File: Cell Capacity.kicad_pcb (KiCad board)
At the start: 2 copper layers, 84.5 x 80.5 mm, 24 parts, among them Q1 IRLZ44N, SW1 SW_Push, SW2 SW_Push, U1 LM358

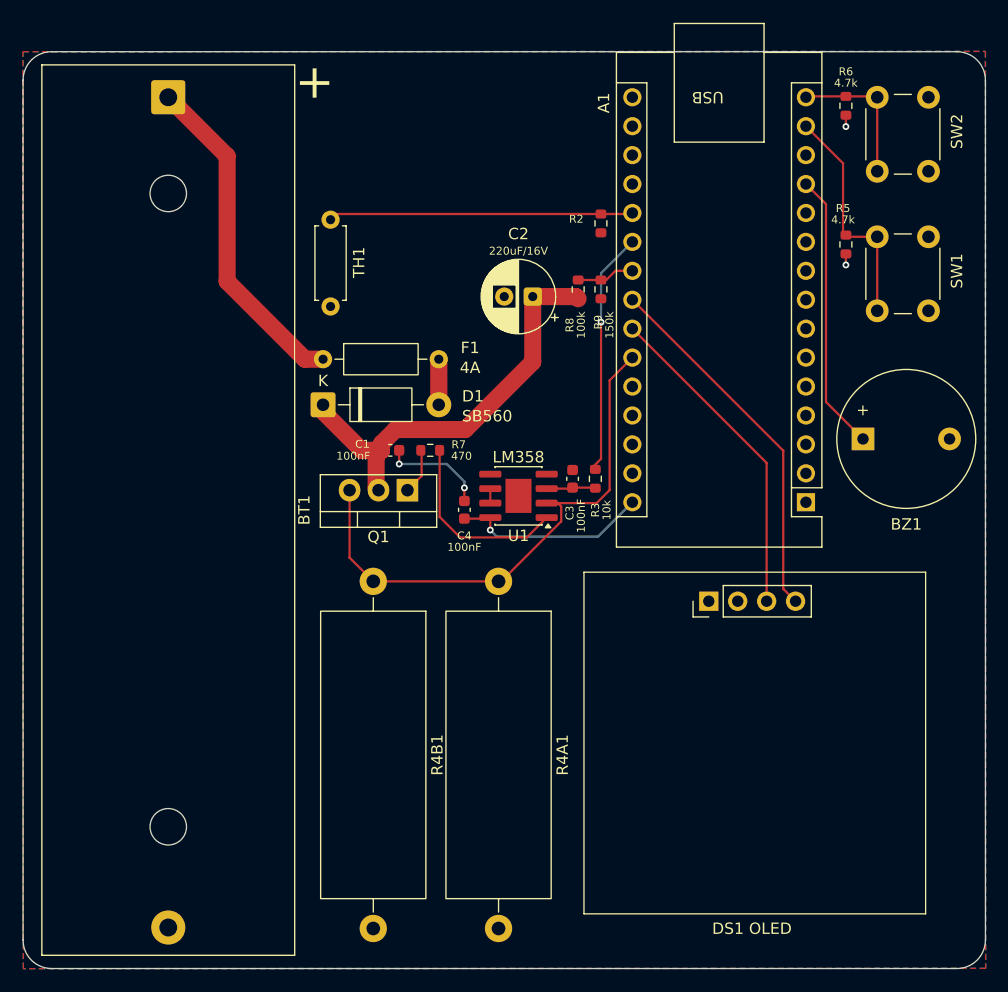
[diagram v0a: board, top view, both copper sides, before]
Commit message: layout iter2
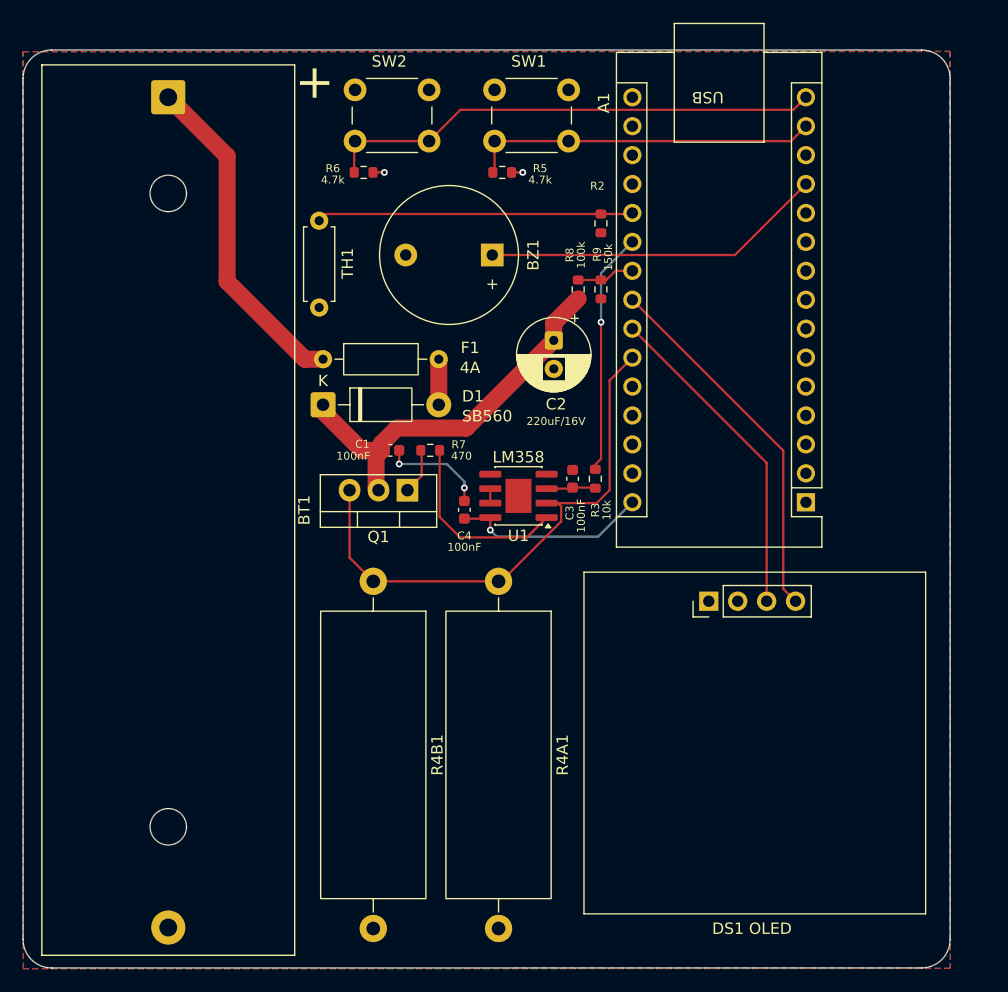
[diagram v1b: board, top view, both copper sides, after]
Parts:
- moved R6 42.8 mm to (94.9, 59.4), turned to 180 degrees
- moved SW2 39.4 mm to (100.7, 56.6), turned to 180 degrees
- moved BZ1 36.3 mm to (106.2, 66.6), turned to 180 degrees
- moved SW1 30.9 mm to (112.9, 56.6), turned to 180 degrees
- moved R5 30.8 mm to (107.1, 59.4), turned to 180 degrees
- moved C2 4.27 mm to (111.6, 74.1), turned to -90 degrees
- moved TH1 1.00 mm to (91.0, 71.2)
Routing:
- net /DOWN: track 12.7 -> 44.0 mm
- net /UP/START: track 20.3 -> 31.0 mm
- net /BUZZ: track 24.5 -> 30.1 mm
- net /batt+: track 37.6 -> 34.9 mm
- net /TEMP: track 26.7 -> 27.8 mm
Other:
- board size 84.5 x 80.5 mm -> 81.4 x 80.6 mm
